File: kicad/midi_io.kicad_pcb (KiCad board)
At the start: 2 copper layers, 38.1 x 41.4 mm, 10 parts, among them J1 MIDI Out, J2 MIDI In, J3 Conn_01x04, U1 6N138

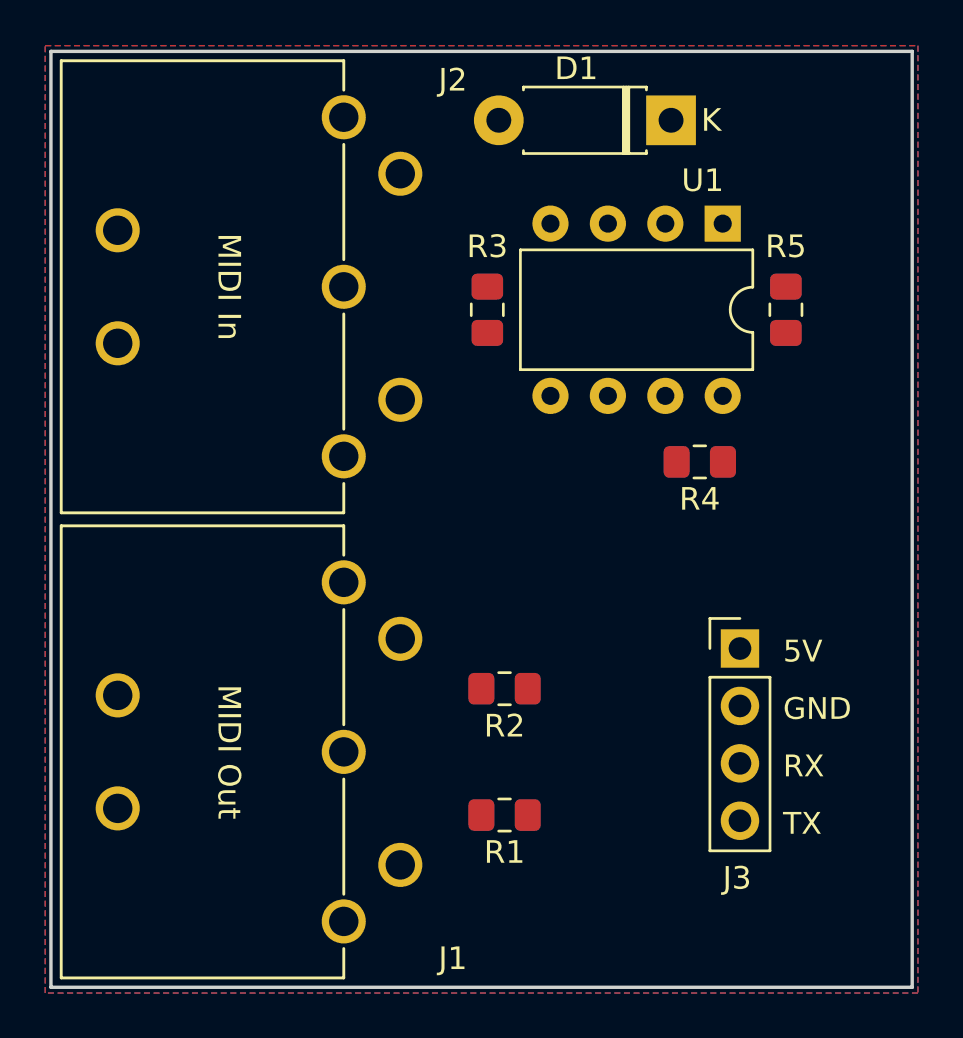
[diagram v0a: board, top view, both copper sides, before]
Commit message: Re-route PCB
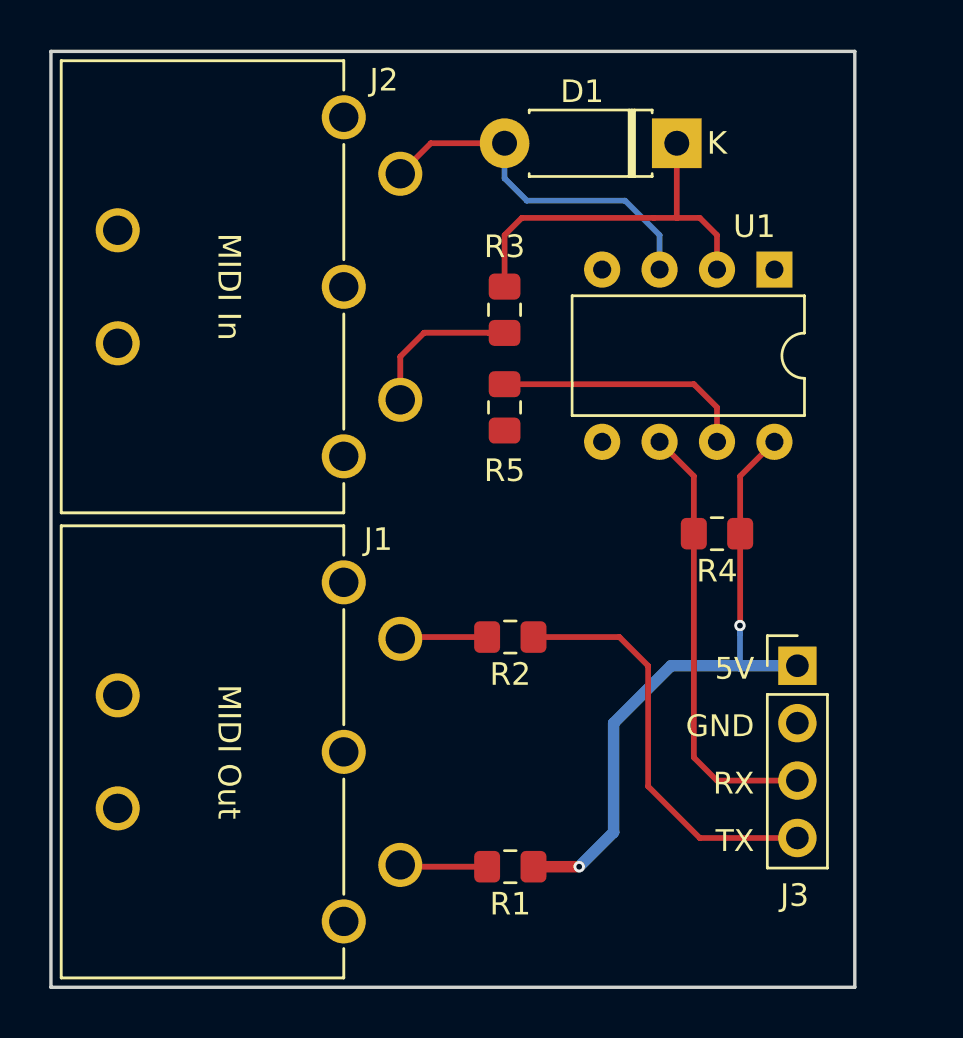
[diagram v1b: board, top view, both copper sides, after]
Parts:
- moved R5 13.2 mm to (131.1, 100.2), turned to 270 degrees
- moved R4 3.27 mm to (140.5, 105.8)
- moved U1 3.06 mm to (143.0, 94.1)
- moved J3 2.65 mm to (144.0, 111.6)
- moved R1 2.30 mm to (131.3, 120.5)
- moved R2 2.30 mm to (131.3, 110.4)
- moved D1 1.05 mm to (138.7, 88.5)
- moved R3 0.76 mm to (131.1, 95.9)
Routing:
- net VCC: track 0.00 -> 28.7 mm, vias 0 -> 2
- net /RX: track 0.00 -> 19.6 mm
- net /TX: track 0.00 -> 18.5 mm
- net Net-(D1-Pad1): track 0.00 -> 17.1 mm
- net Net-(D1-Pad2): track 0.00 -> 16.1 mm
- net Net-(R5-Pad1): track 0.00 -> 11.3 mm
- net Net-(J2-Pad4): track 0.00 -> 6.97 mm
- net Net-(J1-Pad5): track 0.00 -> 3.87 mm
- net Net-(J1-Pad4): track 0.00 -> 3.87 mm
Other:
- board size 38.1 x 41.4 mm -> 35.6 x 41.4 mm
